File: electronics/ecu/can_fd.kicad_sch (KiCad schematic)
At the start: 4 parts, among them U401 ISO1042BQDWVRQ1 (CAN-FD #1 en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, U402 ISO1042BQDWVRQ1 (CAN-FD #2 BO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, U403 ISO1042BQDWVRQ1 (CAN #3 BMS), U404 MCP2518FDT-E/SL

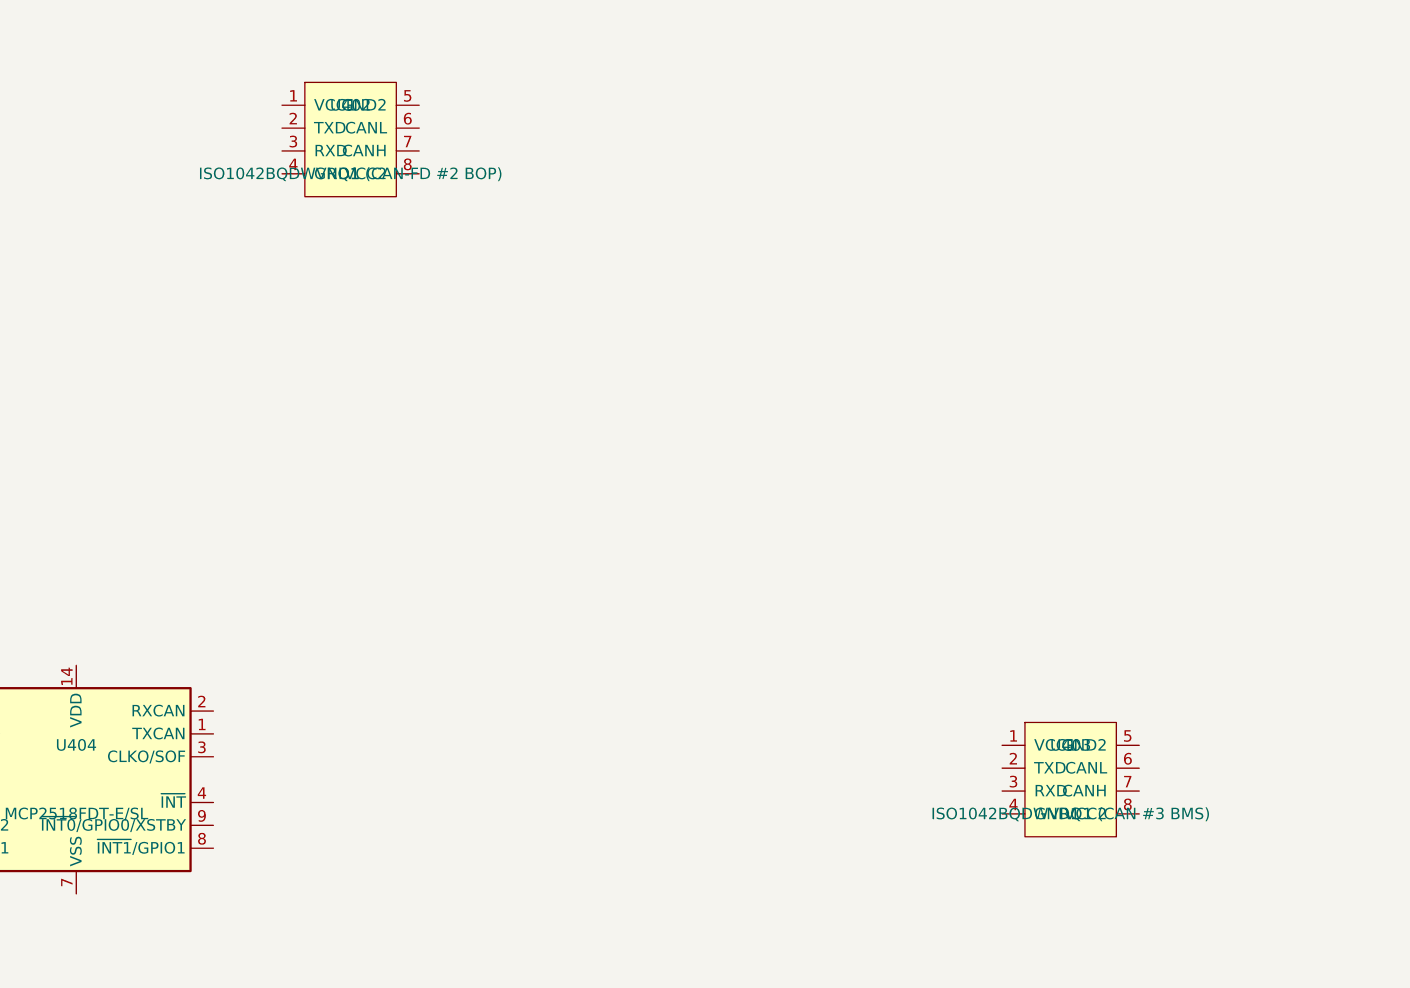
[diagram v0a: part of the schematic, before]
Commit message: WIP: HVAC power modes, fire suppression, insulated-hall recheck; electrical EMS, boards, 3D room model; engine E1–E4 in progress
Co-Authored-By: Claude Fable 5.1 <noreply@anthropic.com>
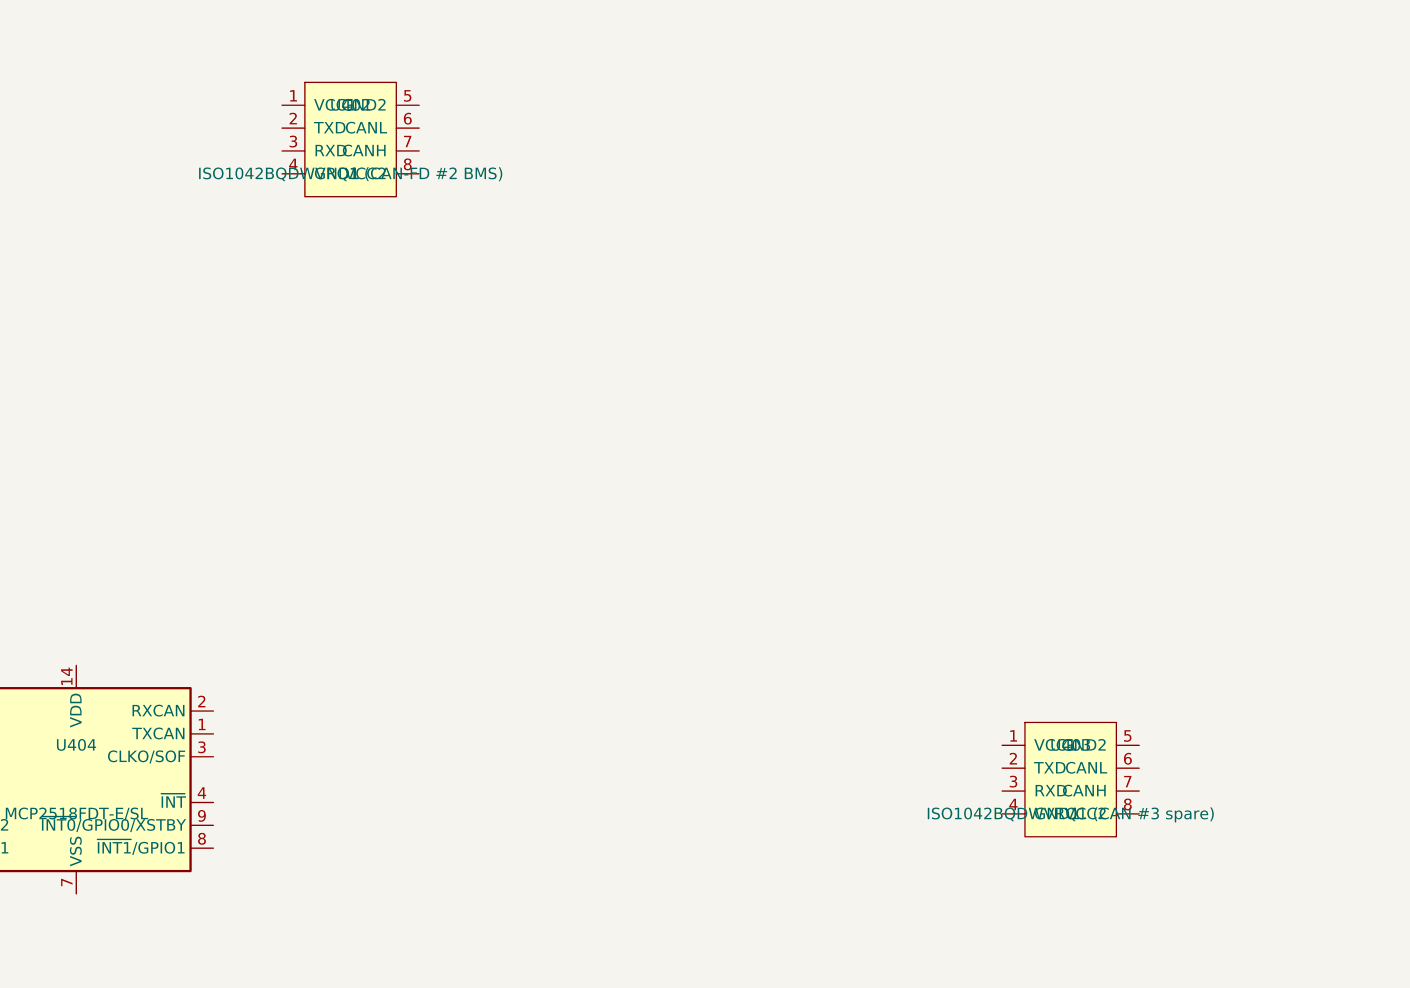
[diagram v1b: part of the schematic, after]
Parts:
- U402: value ISO1042BQDWVRQ1 (CAN-FD #2 BOP) -> ISO1042BQDWVRQ1 (CAN-FD #2 BMS)
- U403: value ISO1042BQDWVRQ1 (CAN #3 BMS) -> ISO1042BQDWVRQ1 (CAN #3 spare)
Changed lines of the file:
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@@
 			(effects (font (size 1.27 1.27)))
 		)
-		(property "Value" "ISO1042BQDWVRQ1 (CAN-FD #2 BOP)"
+		(property "Value" "ISO1042BQDWVRQ1 (CAN-FD #2 BMS)"
 			(at 180.34 123.19 0)
 			(effects (font (size 1.27 1.27)))
@@
 			(effects (font (size 1.27 1.27)))
 		)
-		(property "Value" "ISO1042BQDWVRQ1 (CAN #3 BMS)"
+		(property "Value" "ISO1042BQDWVRQ1 (CAN #3 spare)"
 			(at 260.35 194.31 0)
 			(effects (font (size 1.27 1.27)))
